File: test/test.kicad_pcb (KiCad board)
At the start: 2 copper layers, 16 parts, among them SW1 SW_SPST, U1 LM358P

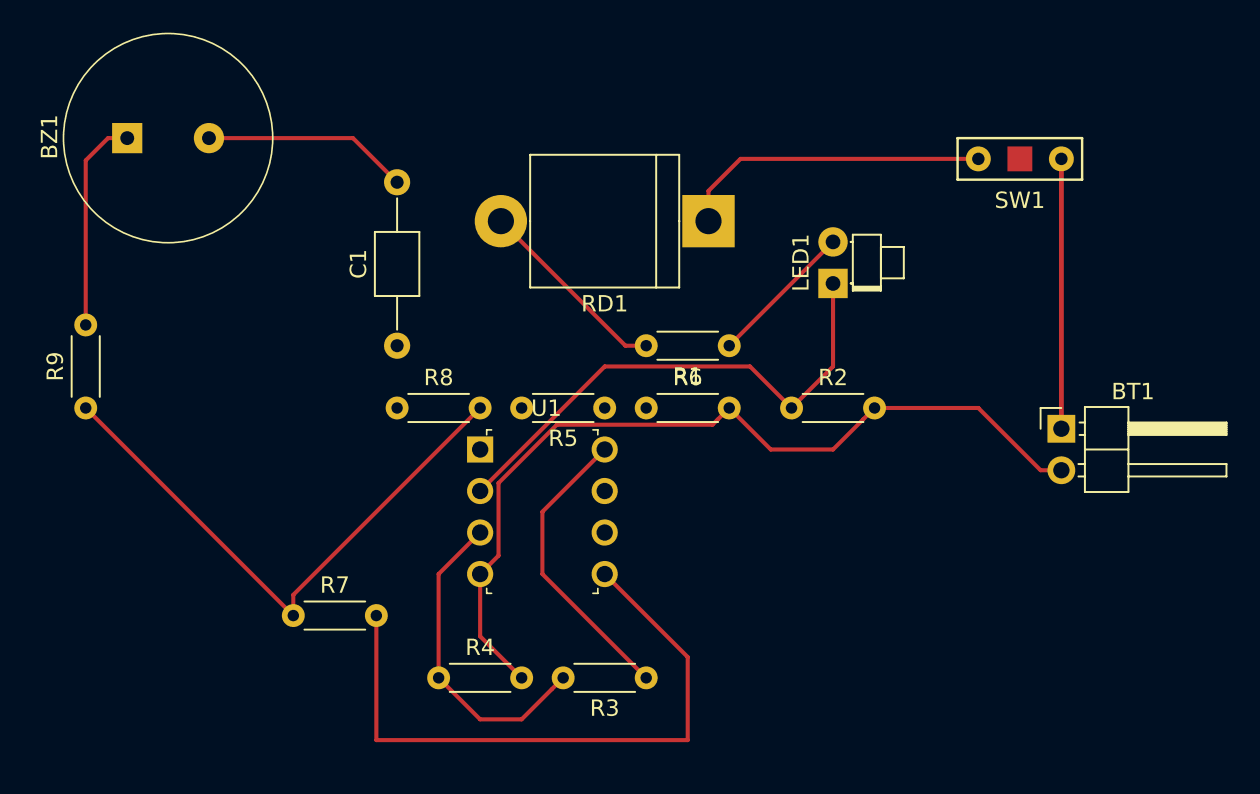
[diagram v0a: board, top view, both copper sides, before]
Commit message: Updated 7/2/20119 during meeting at RRFC
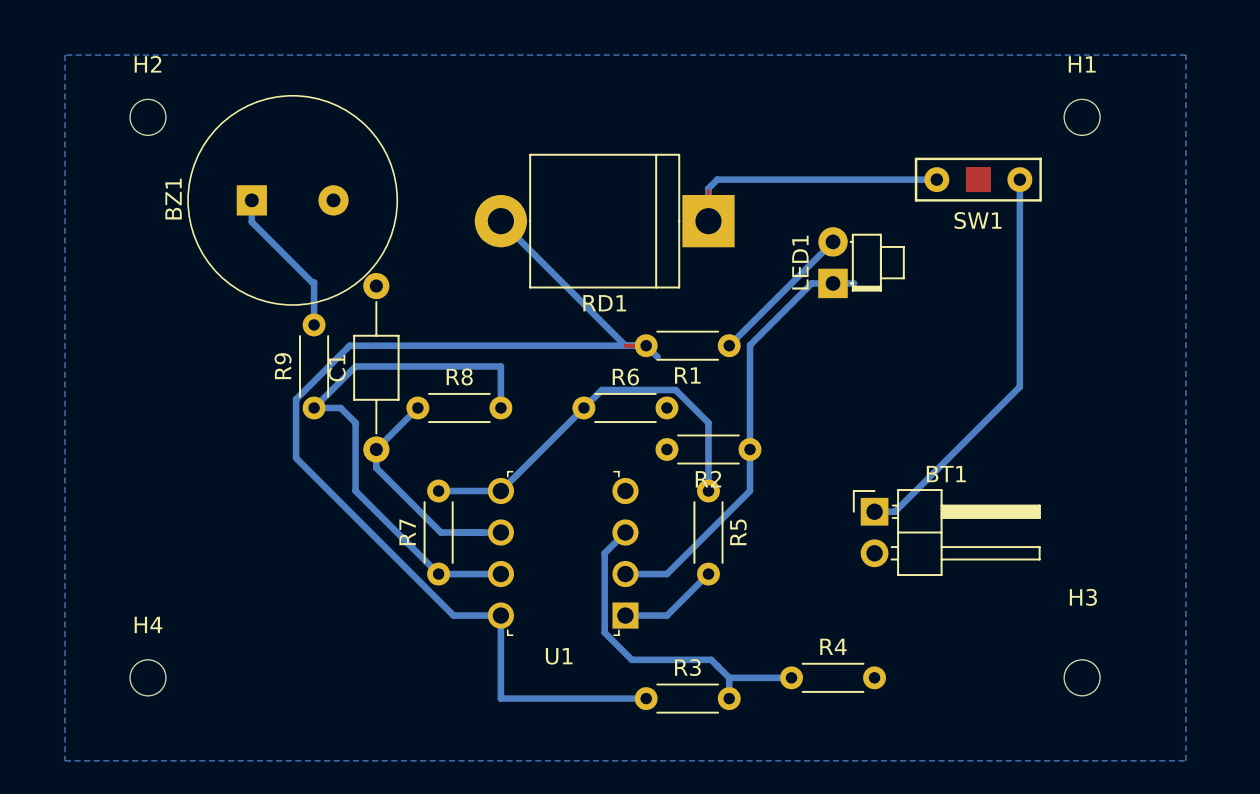
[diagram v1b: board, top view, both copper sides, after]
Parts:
- added H1: MountingHole, MountingHole:MountingHole_2.2mm_M2, F.Cu at (184.2, 91.4)
- added H2: MountingHole, MountingHole:MountingHole_2.2mm_M2, F.Cu at (127.0, 91.4)
- added H3: MountingHole, MountingHole:MountingHole_2.2mm_M2, F.Cu at (184.2, 125.7)
- added H4: MountingHole, MountingHole:MountingHole_2.2mm_M2, F.Cu at (127.0, 125.7)
- moved R4 21.6 mm to (166.4, 125.7)
- moved R9 14.0 mm to (137.2, 109.2)
- moved U1 13.5 mm to (156.2, 121.9), turned to 180 degrees
- moved BT1 12.5 mm to (171.4, 115.6)
- moved R7 9.25 mm to (144.8, 119.4), turned to 90 degrees
- moved BZ1 8.52 mm to (133.3, 96.5)
- moved R5 8.13 mm to (161.3, 114.3), turned to 270 degrees
- moved C1 6.48 mm to (141.0, 111.8)
- moved R6 3.81 mm to (153.7, 109.2)
- moved R2 3.59 mm to (163.8, 111.8), turned to 180 degrees
- moved SW1 2.84 mm to (177.8, 95.2)
- moved R3 1.27 mm to (157.5, 127.0), turned to 0 degrees
- moved R8 1.27 mm to (143.5, 109.2)
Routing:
- net GND: track 66.1 -> 0.00 mm
- net Net-(R1-Pad2): track 30.2 -> 71.2 mm
- net Net-(C1-Pad1): track 0.00 -> 15.7 mm
- net Net-(R5-Pad1): track 38.9 -> 24.1 mm
- net +9V: track 33.0 -> 24.7 mm
- net Net-(R5-Pad2): track 0.00 -> 6.13 mm
- net Net-(LED1-Pad1): track 31.9 -> 26.6 mm
- net Net-(BZ1-Pad1): track 13.2 -> 9.26 mm
- net /Link: track 35.4 -> 33.1 mm
- net Net-(RD1-Pad1): track 19.2 -> 18.0 mm
- net Net-(R3-Pad2): track 19.7 -> 20.5 mm
- added copper zone on B.Cu, net GND
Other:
- net class Default: trace_width 0.25 -> 0.4
